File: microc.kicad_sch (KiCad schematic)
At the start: 11 parts, among them SW1 SW_SPST

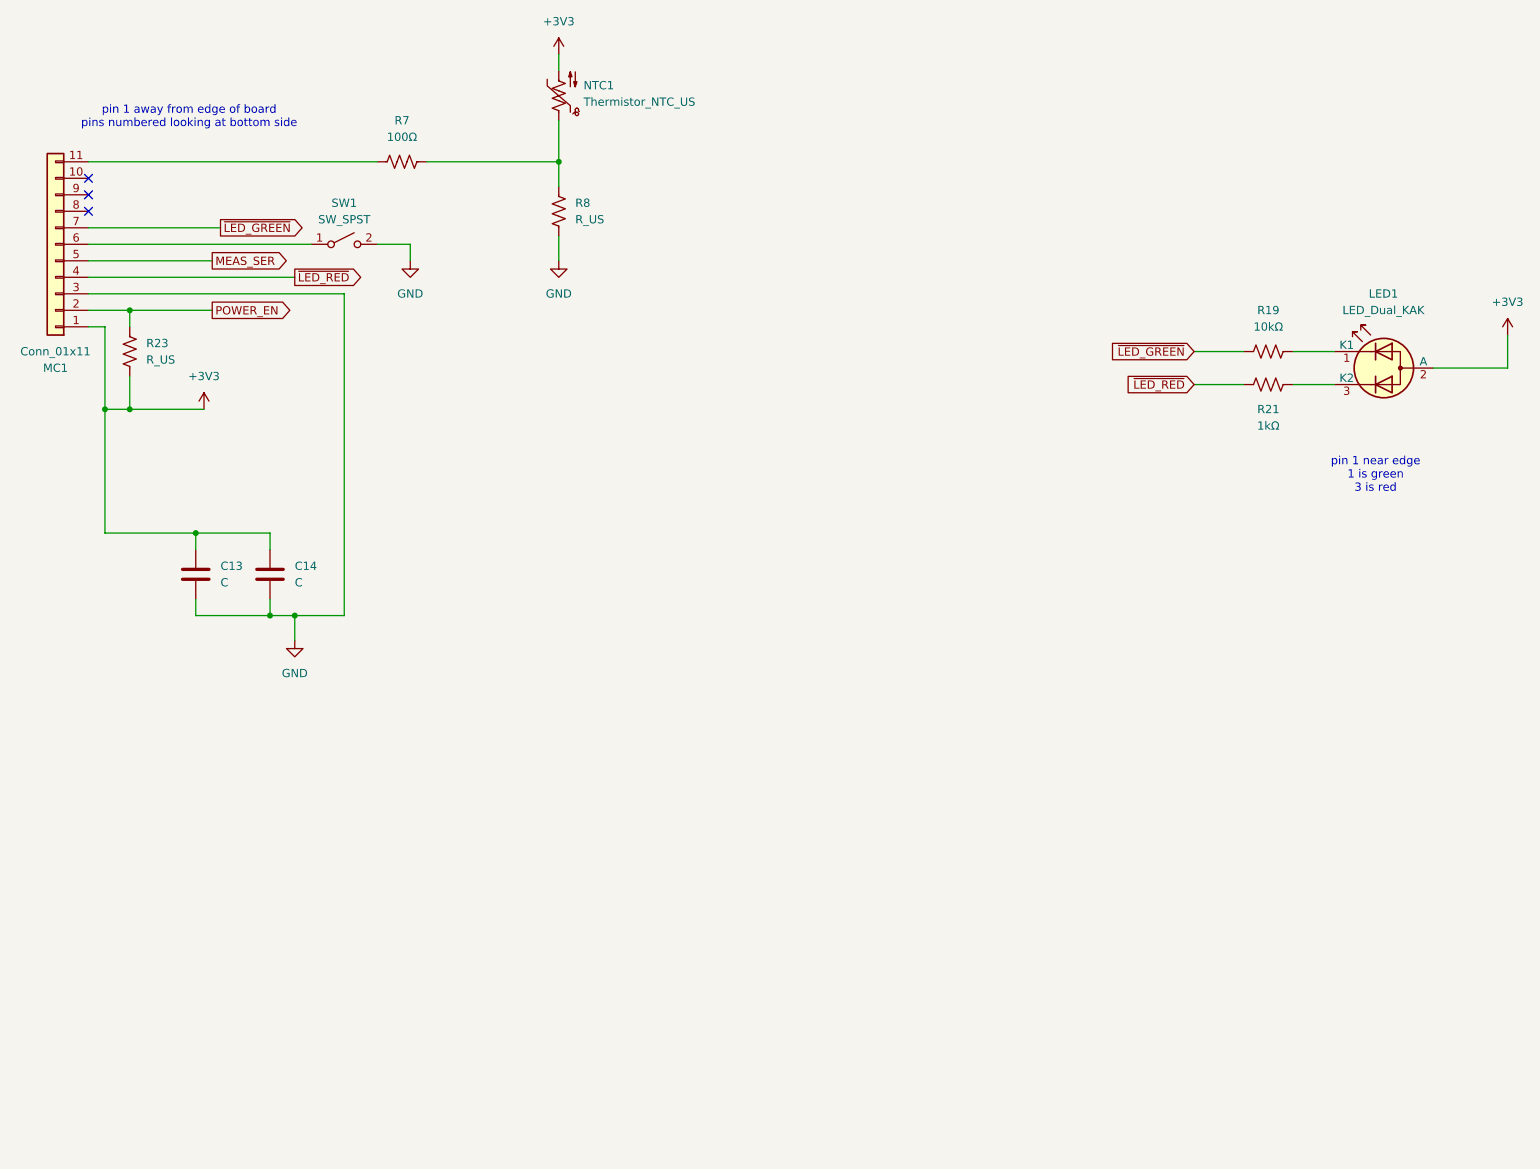
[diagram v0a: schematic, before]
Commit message: Cleaning up layout
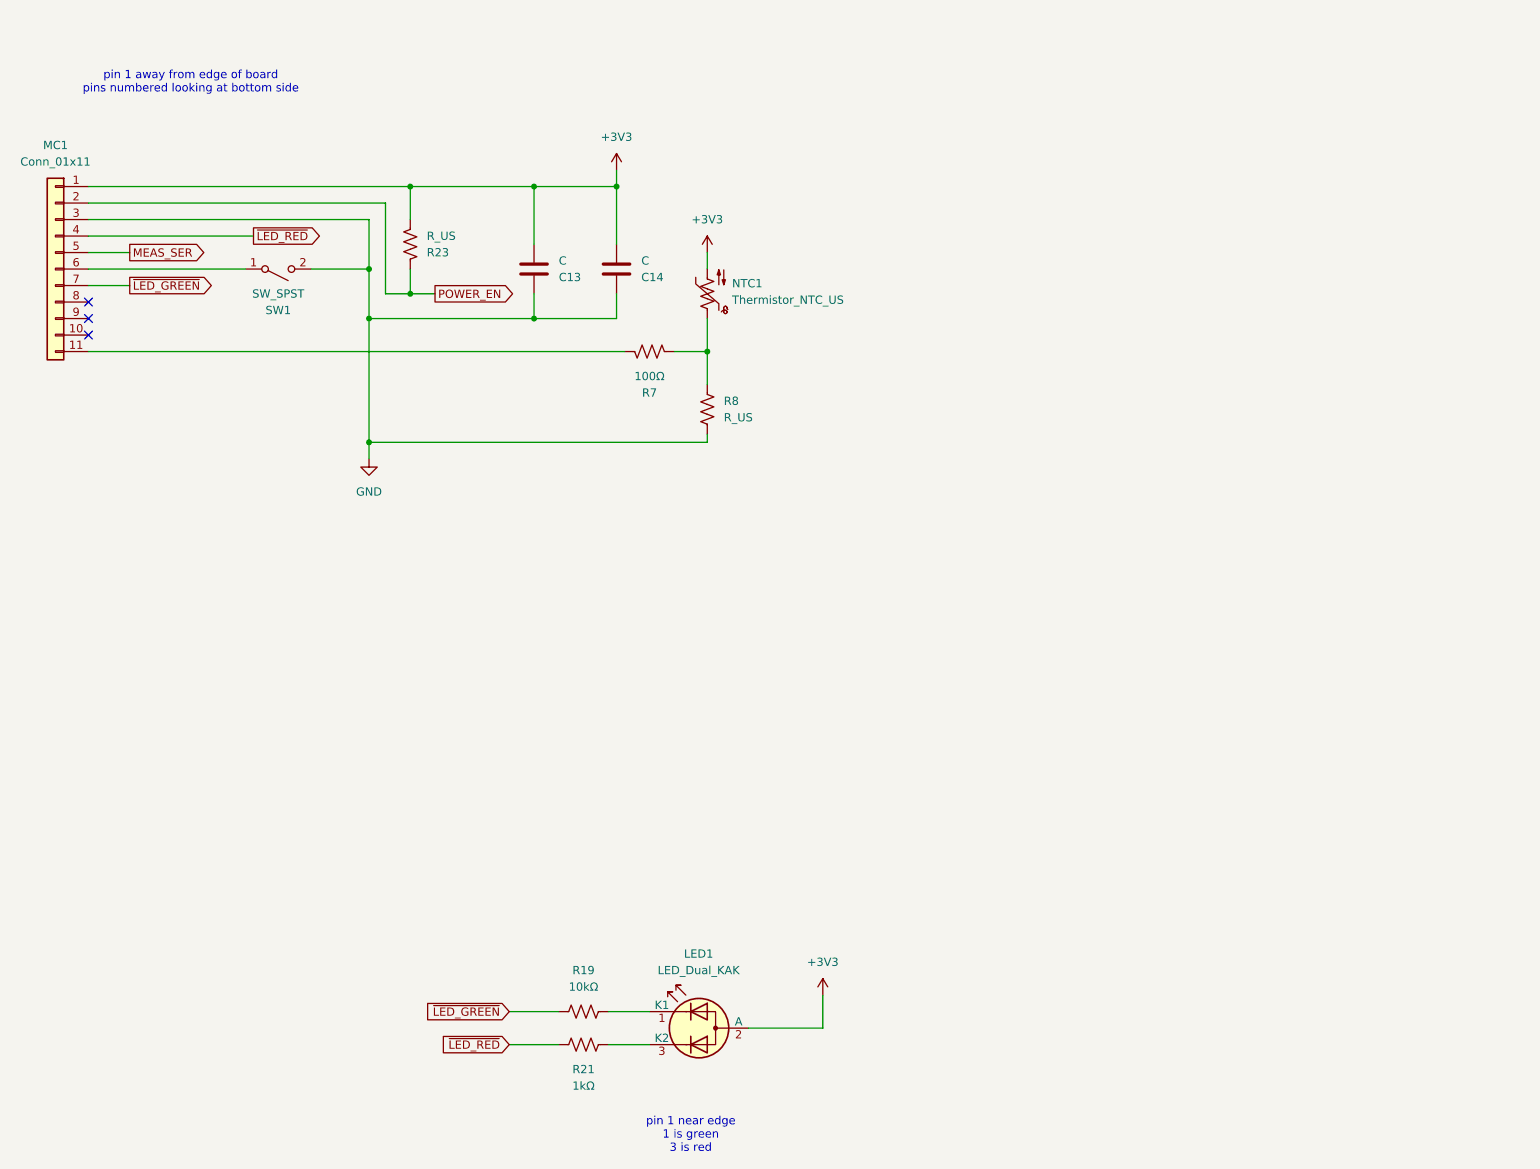
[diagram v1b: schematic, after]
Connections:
- net +3V3: now also C13.2, C14.2; no longer C13.1, C14.1
- net GND: now also C13.1, C14.1; no longer C13.2, C14.2
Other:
- moved on the sheet: C13, C14, LED1, MC1, NTC1, R19, R21, R23, R7, R8, SW1
